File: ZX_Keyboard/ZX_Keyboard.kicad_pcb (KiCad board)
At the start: 2 copper layers, 101.6 x 50.8 mm, 132 parts, among them J1 DBG_UART, J2 BOOT2, J3 SWD, J4 BOOT, SW1 RESET, U1 STM32F105R8Tx, Y1 8MHz

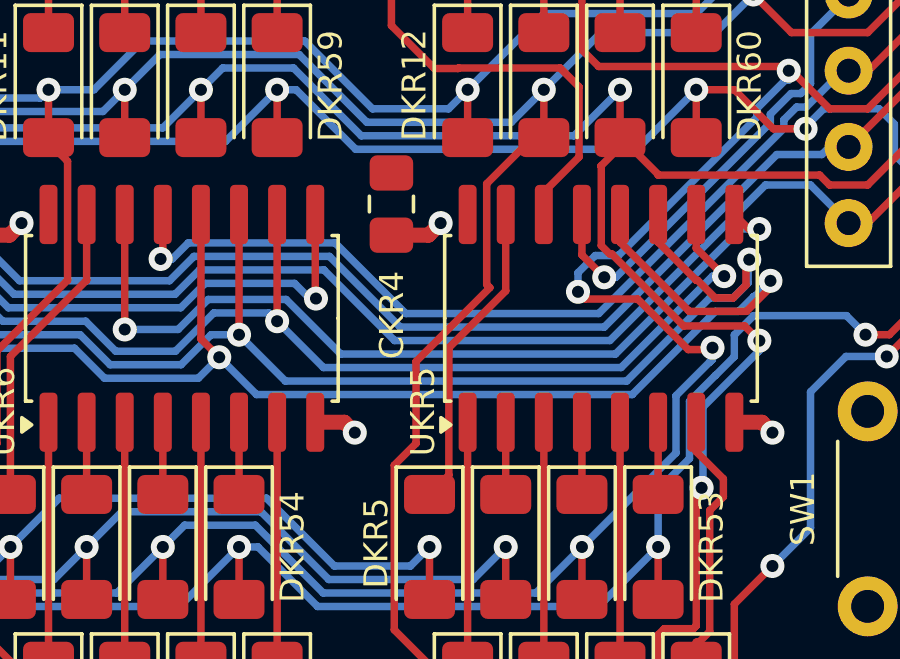
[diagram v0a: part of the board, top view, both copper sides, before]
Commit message: update Schematic and PCB
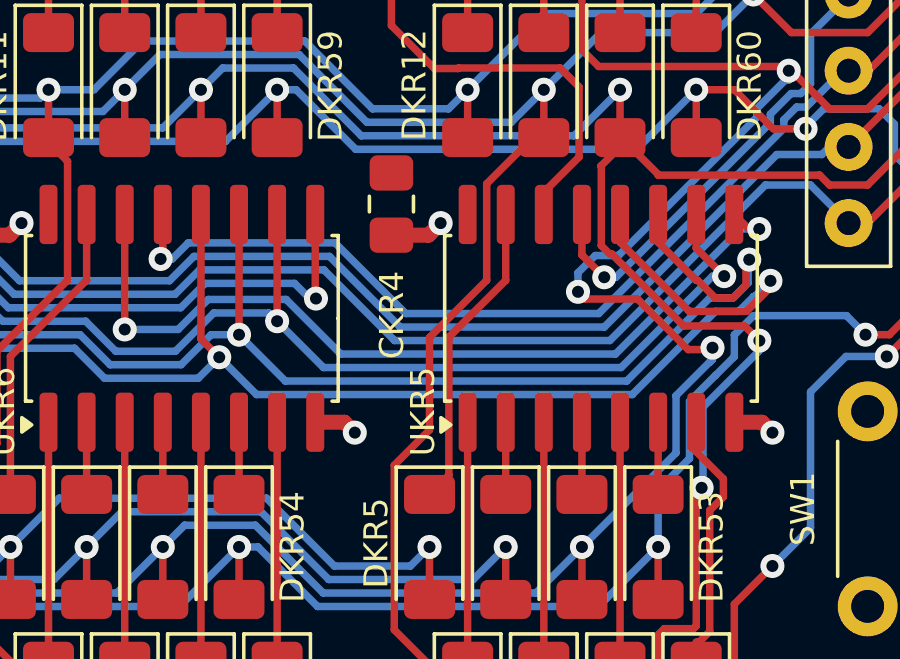
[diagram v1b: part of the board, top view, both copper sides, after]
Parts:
- C8, CKR3, CKR8: value 4.7uFx6.3V -> 4,7uFx6,3V
- CC2: value 4,7uFx6.3V -> 4,7uFx6,3V
- CPS1, CPS4: value 10uFx6.3v -> 10uFx6,3v
